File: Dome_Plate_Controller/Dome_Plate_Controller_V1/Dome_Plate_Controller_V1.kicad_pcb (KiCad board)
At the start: 4 copper layers, 118 x 78.6 mm, 43 parts, among them J1 USB_B_Micro, J10 SERIAL_FU4, J11 SERIAL_FU3, J12 SERIAL_FU, J13 DB25_Female_MagTag, J14 DC-005-5A-2.0, J15 SERIAL_FU2, J2 DB25_Male_SlipRing, J3 12VOUT, J4 SERIAL_RS, J5 12OUT, J6 12VOUT, J7 5V OUT, J8 5V Out 2, J9 5V Out, SW1 SW_Push, U1 ESP32-WROOM-32D_16MB_, U2 CJ2301_S1, U3 ME6211C33M5G, U4 CH340C, U5 UMH3N, U6 D36V50F5-STEPDOWN

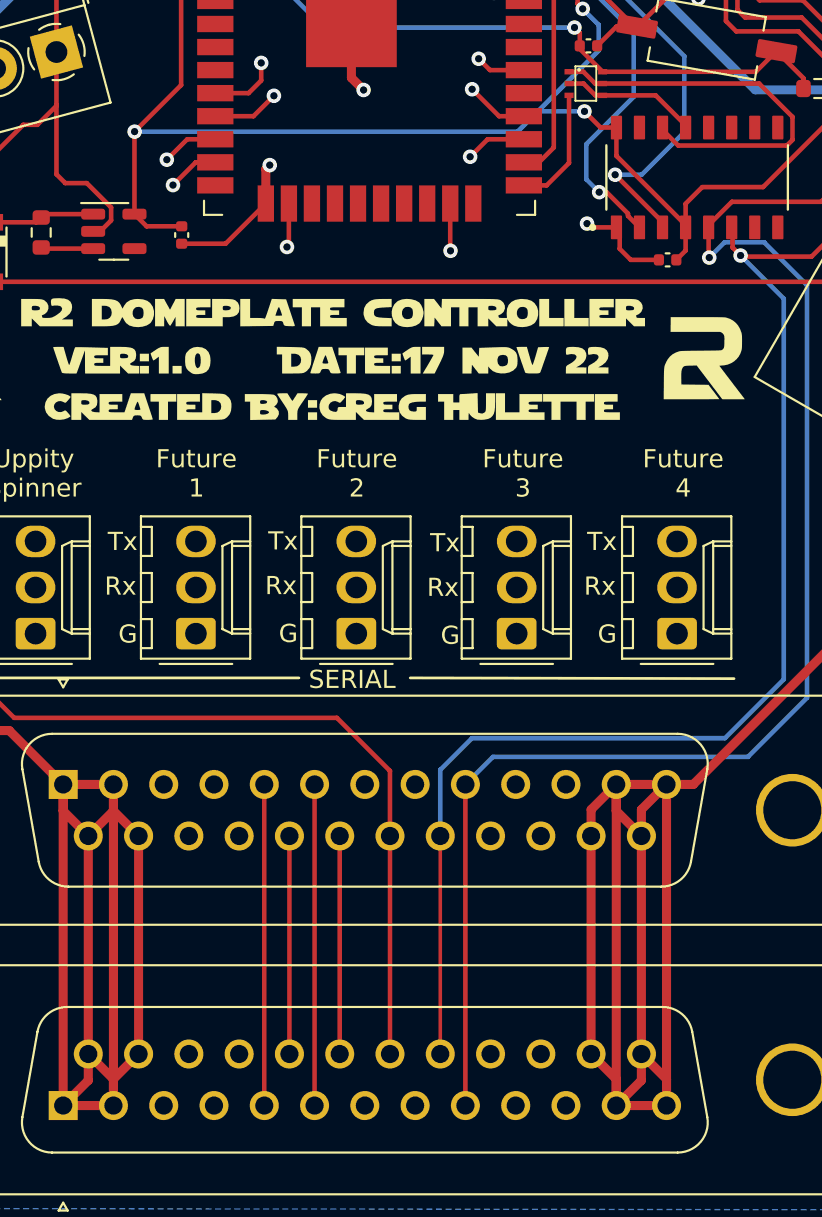
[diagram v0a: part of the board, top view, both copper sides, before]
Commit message: Added a lot since last check in
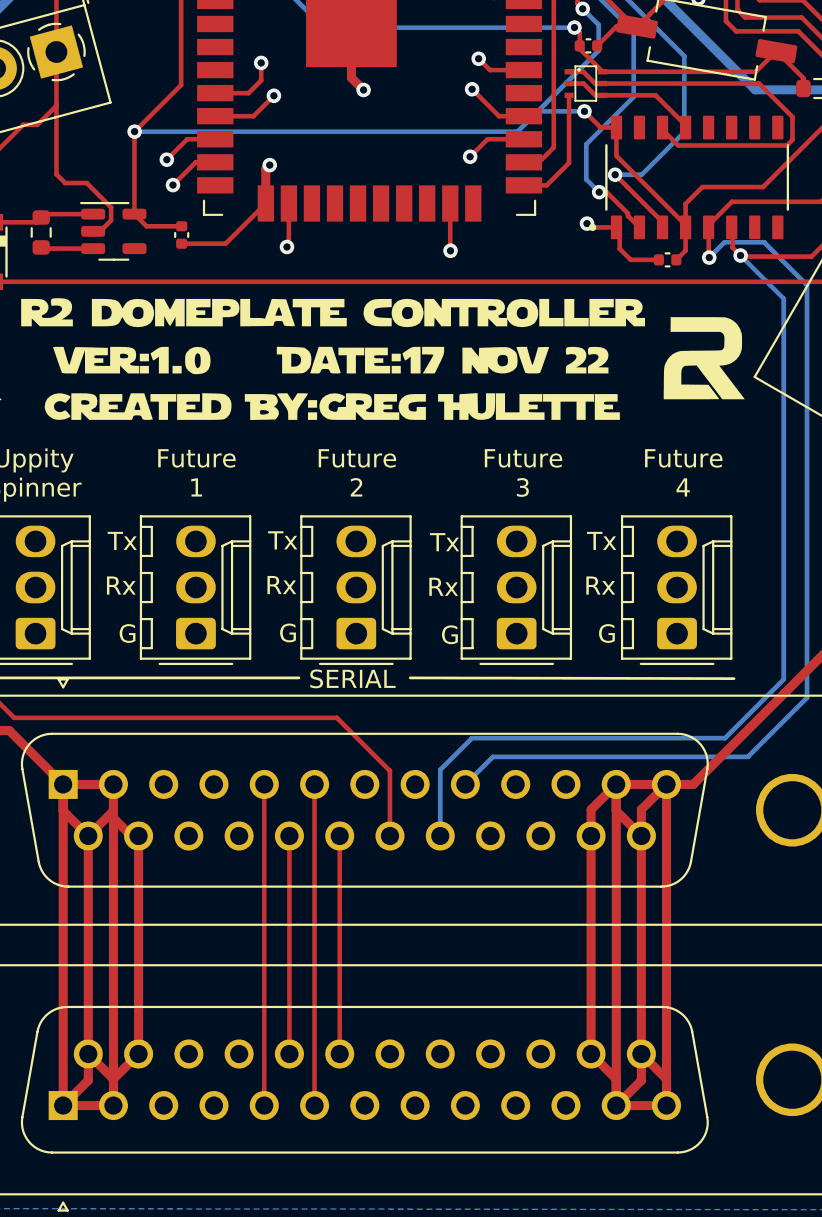
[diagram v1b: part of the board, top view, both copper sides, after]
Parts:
- J4: value SERIAL_RS -> SERIAL_US
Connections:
- J13 pad 20: VBUS -> unconnected-(J13-Pad20)
- J13 pad 21: D- -> unconnected-(J13-Pad21)
- J13 pad 8: GND -> unconnected-(J13-Pad8)
- J13 pad 9: D+ -> unconnected-(J13-Pad9)
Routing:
- net +12V: track 257.8 -> 510.7 mm
- net unconnected-(J2-Pad0): track 0.00 -> 53.2 mm
- net unconnected-(J13-Pad0): track 0.00 -> 51.6 mm
- net D+: track 95.6 -> 77.8 mm
- net VBUS: track 143.8 -> 131.8 mm
- net D-: track 89.0 -> 76.9 mm

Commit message: added LED PCBs
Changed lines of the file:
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@@
       (drillshape 0)
       (scaleselection 1)
-      (outputdirectory "Gerber/Dome_ControllerV2.0/")
+      (outputdirectory "BOM and CPL/")
     )
   )
@@
     (fp_line (start -1.27 -0.5) (end -0.562893 0) (layer "F.Fab") (width 0.1))
     (fp_line (start -1.27 2.88) (end 6.35 2.88) (layer "F.Fab") (width 0.1))
-    (pad "1" thru_hole roundrect locked (at 0 0 90) (size 1.74 2.19) (drill 1.19) (layers *.Cu *.Mask) (roundrect_rratio 0.143678)
+    (pad "1" thru_hole roundrect locked (at 0 0 90) (size 1.74 2.19) (drill 1.19) (layers *.Cu *.Mask) (roundrect_rratio 0.1436781609)
       (net 2 "GND") (pinfunction "Pin_1") (pintype "passive"))
     (pad "2" thru_hole oval locked (at 2.54 0 90) (size 1.74 2.19) (drill 1.19) (layers *.Cu *.Mask)
@@
     (fp_line (start 6.35 -2.92) (end -1.27 -2.92) (layer "F.Fab") (width 0.1))
     (fp_line (start 6.35 2.88) (end 6.35 -2.92) (layer "F.Fab") (width 0.1))
-    (pad "1" thru_hole roundrect locked (at 0 0 90) (size 1.74 2.19) (drill 1.19) (layers *.Cu *.Mask) (roundrect_rratio 0.143678)
+    (pad "1" thru_hole roundrect locked (at 0 0 90) (size 1.74 2.19) (drill 1.19) (layers *.Cu *.Mask) (roundrect_rratio 0.1436781609)
       (net 2 "GND") (pinfunction "Pin_1") (pintype "passive"))
     (pad "2" thru_hole oval locked (at 2.54 0 90) (size 1.74 2.19) (drill 1.19) (layers *.Cu *.Mask)
@@
     (fp_line (start -1.27 -2.92) (end -1.27 2.88) (layer "F.Fab") (width 0.1))
     (fp_line (start 6.35 -2.92) (end -1.27 -2.92) (layer "F.Fab") (width 0.1))
-    (pad "1" thru_hole roundrect locked (at 0 0 90) (size 1.74 2.19) (drill 1.19) (layers *.Cu *.Mask) (roundrect_rratio 0.143678)
+    (pad "1" thru_hole roundrect locked (at 0 0 90) (size 1.74 2.19) (drill 1.19) (layers *.Cu *.Mask) (roundrect_rratio 0.1436781609)
       (net 2 "GND") (pinfunction "Pin_1") (pintype "passive"))
     (pad "2" thru_hole oval locked (at 2.54 0 90) (size 1.74 2.19) (drill 1.19) (layers *.Cu *.Mask)
@@
     (fp_line (start 6.35 2.88) (end 6.35 -2.92) (layer "F.Fab") (width 0.1))
     (fp_line (start -1.27 -2.92) (end -1.27 2.88) (layer "F.Fab") (width 0.1))
-    (pad "1" thru_hole roundrect locked (at 0 0 90) (size 1.74 2.19) (drill 1.19) (layers *.Cu *.Mask) (roundrect_rratio 0.143678)
+    (pad "1" thru_hole roundrect locked (at 0 0 90) (size 1.74 2.19) (drill 1.19) (layers *.Cu *.Mask) (roundrect_rratio 0.1436781609)
       (net 2 "GND") (pinfunction "Pin_1") (pintype "passive"))
     (pad "2" thru_hole oval locked (at 2.54 0 90) (size 1.74 2.19) (drill 1.19) (layers *.Cu *.Mask)
@@
     (fp_line (start -1.27 -0.5) (end -0.562893 0) (layer "F.Fab") (width 0.1))
     (fp_line (start -1.27 2.88) (end 6.35 2.88) (layer "F.Fab") (width 0.1))
-    (pad "1" thru_hole roundrect locked (at 0 0 90) (size 1.74 2.19) (drill 1.19) (layers *.Cu *.Mask) (roundrect_rratio 0.143678)
+    (pad "1" thru_hole roundrect locked (at 0 0 90) (size 1.74 2.19) (drill 1.19) (layers *.Cu *.Mask) (roundrect_rratio 0.1436781609)
       (net 2 "GND") (pinfunction "Pin_1") (pintype "passive"))
     (pad "2" thru_hole oval locked (at 2.54 0 90) (size 1.74 2.19) (drill 1.19) (layers *.Cu *.Mask)
